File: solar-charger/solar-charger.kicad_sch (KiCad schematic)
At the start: 11 parts, among them IC1 TLV809EA30DBZR, IC2 TLV803EB33VDBZR, J1 Conn_01x02_Socket, J2 Conn_01x02_Socket, J3 Conn_01x02_Socket, Q1 AO3415, Q2 AO3416

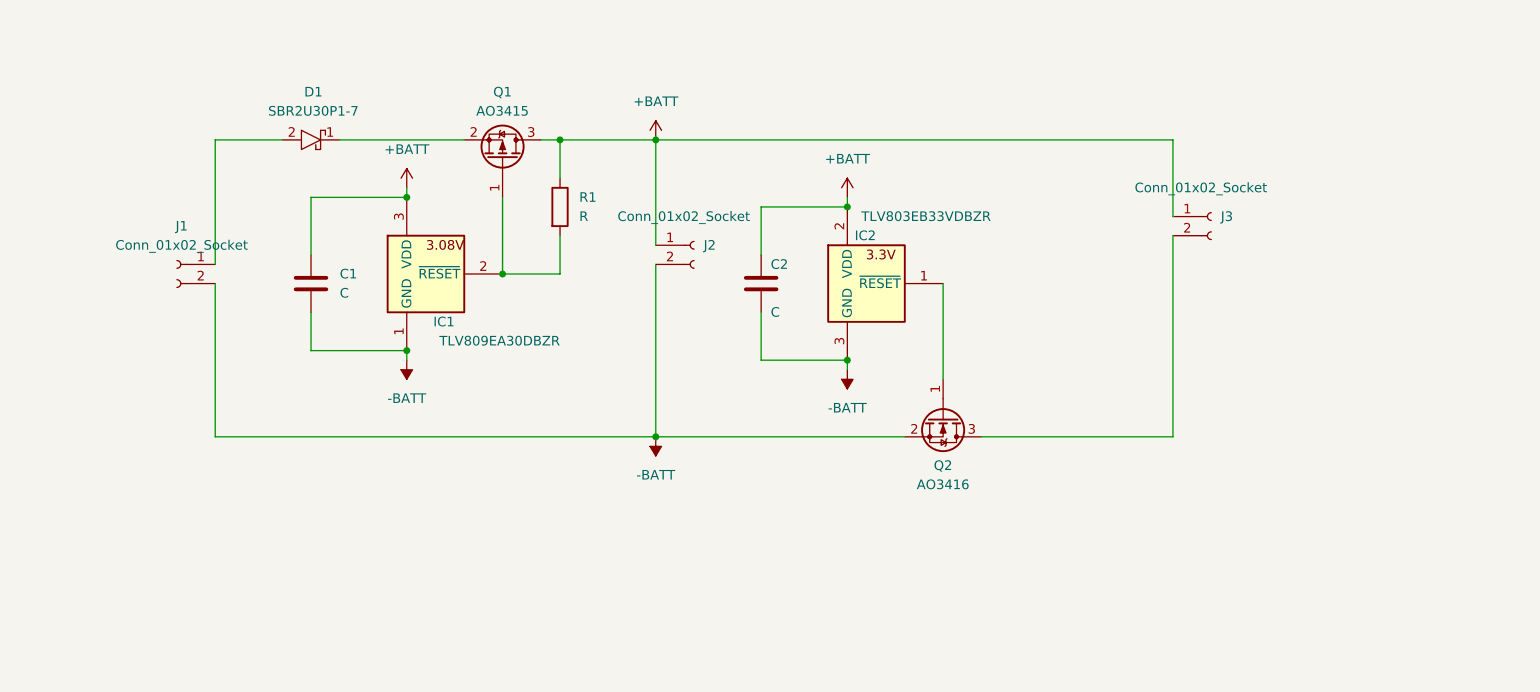
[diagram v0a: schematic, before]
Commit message: finish 1. working PCB
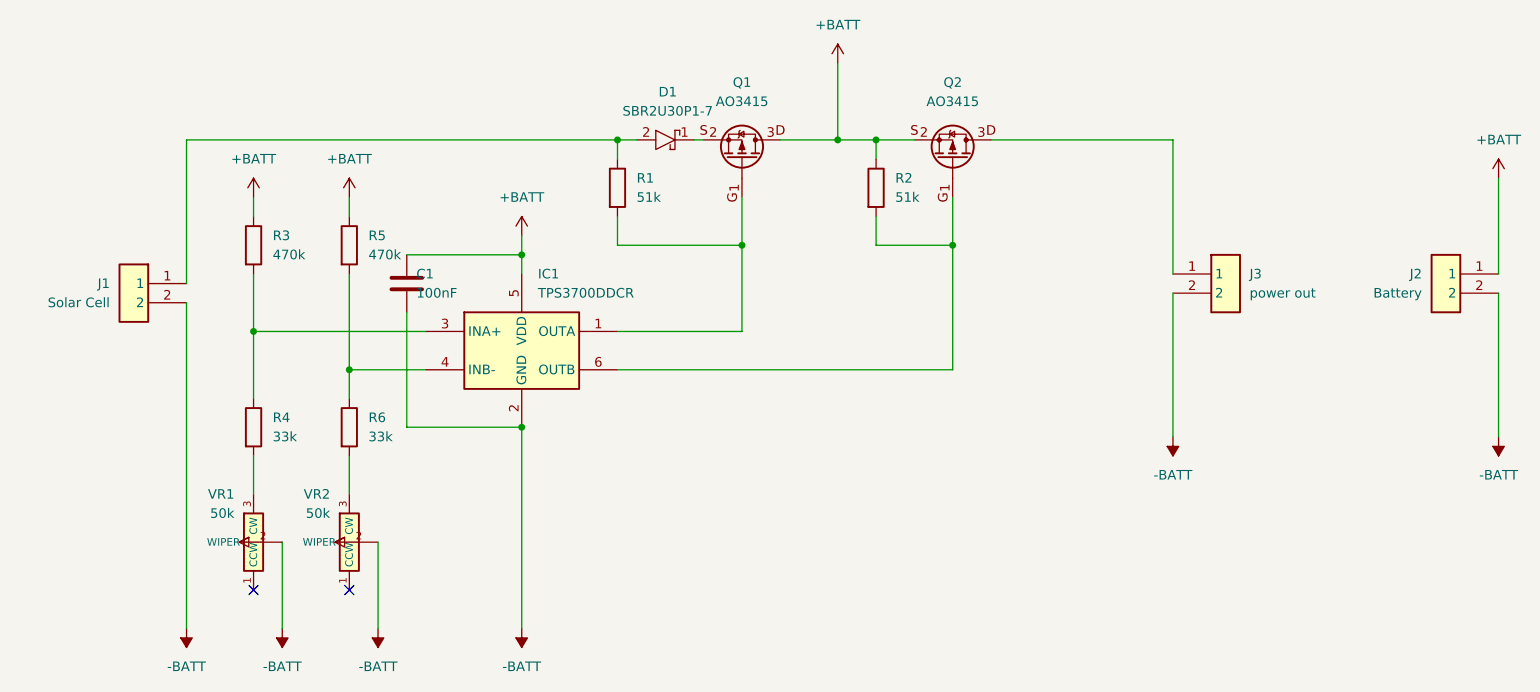
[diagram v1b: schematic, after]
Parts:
- removed C2: C, Capacitor_SMD:C_0805_2012Metric_Pad1.18x1.45mm_HandSolder, symbol Device:C
- removed IC1: TLV809EA30DBZR, Marcus_Library:SOT95P237X95-3N, symbol Marcus-PCB-Library:TLV809EA30DBZR
- removed IC2: TLV803EB33VDBZR, Marcus_Library:SOT95P237X112-3N, symbol Marcus-PCB-Library:TLV803EB33VDBZR
- removed J1, J2, J3: Conn_01x02_Socket, Connector_PinHeader_1.27mm:PinHeader_1x02_P1.27mm_Vertical, symbol Connector:Conn_01x02_Socket
- removed Q2: AO3416, Package_TO_SOT_SMD:SOT-23, symbol Marcus-PCB-Library:AO3416
- added IC1: TPS3700DDCR, Marcus-PCB-Library:SOT98P280X110-6N, symbol Marcus-PCB-Library:TPS3700DDCR
- added J1: Solar Cell, Marcus-PCB-Library:10129378902001BLF, symbol Marcus-PCB-Library:2x-Header-Pin-Through-Hole
- added J2: Battery, Marcus-PCB-Library:10129378902001BLF, symbol Marcus-PCB-Library:2x-Header-Pin-Through-Hole
- added J3: power out, Marcus-PCB-Library:10129378902001BLF, symbol Marcus-PCB-Library:2x-Header-Pin-Through-Hole
- added Q2: AO3415, Package_TO_SOT_SMD:SOT-23, symbol Marcus-PCB-Library:AO3415
- added R2: 51k, Resistor_SMD:R_0805_2012Metric_Pad1.20x1.40mm_HandSolder, symbol Device:R
- added R3, R5: 470k, Resistor_SMD:R_0805_2012Metric_Pad1.20x1.40mm_HandSolder, symbol Device:R
- added R4, R6: 33k, Resistor_SMD:R_0805_2012Metric_Pad1.20x1.40mm_HandSolder, symbol Device:R
- added VR1, VR2: 50k, Marcus-PCB-Library:TC33X2104E, symbol Marcus-PCB-Library:TC33X-trimmer
- C1: value C -> 100nF
- Q1: footprint SOT95P280X125-3N -> Package_TO_SOT_SMD:SOT-23
- R1: value R -> 51k
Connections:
- net +BATT: now also IC1.5 (VDD), J2.1, Q2.2 (S), R2.1, R3.1, R5.1; no longer R1.1
- net -BATT: now also IC1.2 (GND), J1.2, J2.2, J3.2, VR1.2 (WIPER), VR2.2 (WIPER)
- net at D1.2 (A): now also R1.1, J1.1
- net at Q1.1 (G), R1.2: now also IC1.1 (OUTA)
- new net: J3.1, Q2.3 (D)
- new net: IC1.3 (INA+), R3.2, R4.1
- new net: IC1.6 (OUTB), Q2.1 (G), R2.2
- new net: R4.2, VR1.3 (CW)
- new net: IC1.4 (INB-), R5.2, R6.1
- new net: R6.2, VR2.3 (CW)
- no-connect marks 0 -> 2
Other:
- moved on the sheet: C1, D1
